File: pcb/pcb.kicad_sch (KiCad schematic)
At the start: 18 parts, among them J1 USB_C_Receptacle_USB2.0_16P, SW1 SW_Push, U1 USBLC6-2SC6, U2 XC6206PxxxMR, U3 STM32F072CBTx

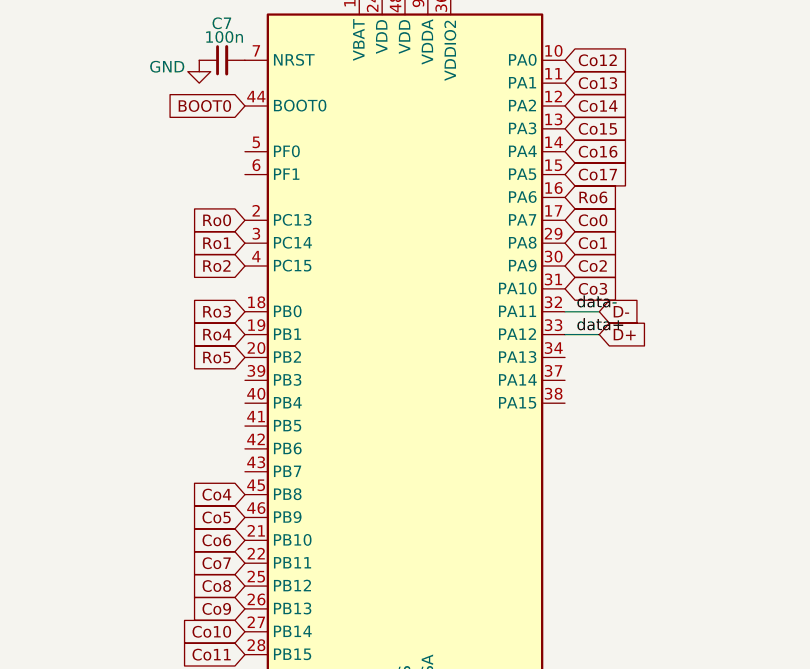
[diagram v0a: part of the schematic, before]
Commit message: Matrix ready
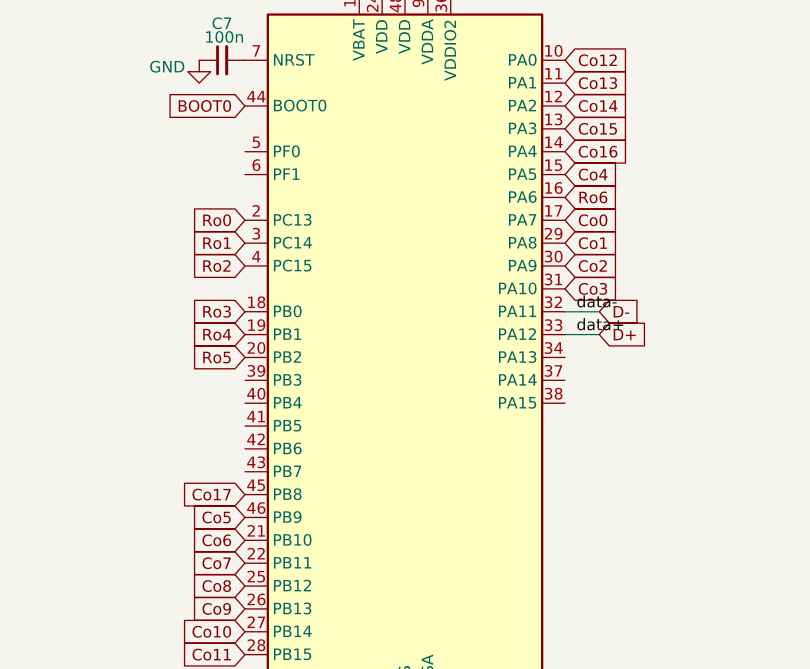
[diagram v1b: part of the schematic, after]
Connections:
- net Co17: now also U3.45 (PB8); no longer U3.15 (PA5)
- net Co4: now also U3.15 (PA5); no longer U3.45 (PB8)
